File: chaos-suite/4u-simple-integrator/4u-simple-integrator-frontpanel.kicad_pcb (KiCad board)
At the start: 2 copper layers, 25 x 175 mm, 1 part

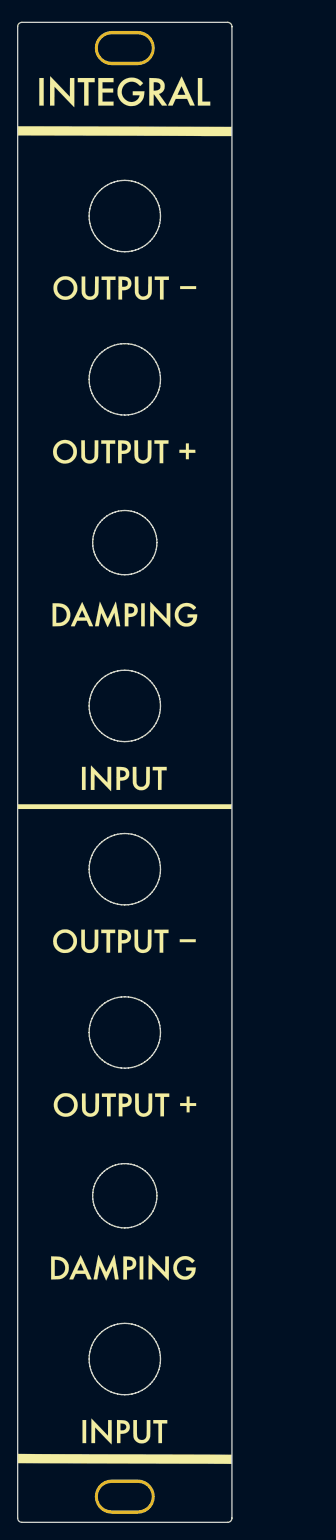
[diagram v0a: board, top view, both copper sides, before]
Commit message: Updating simple integrator to rev2
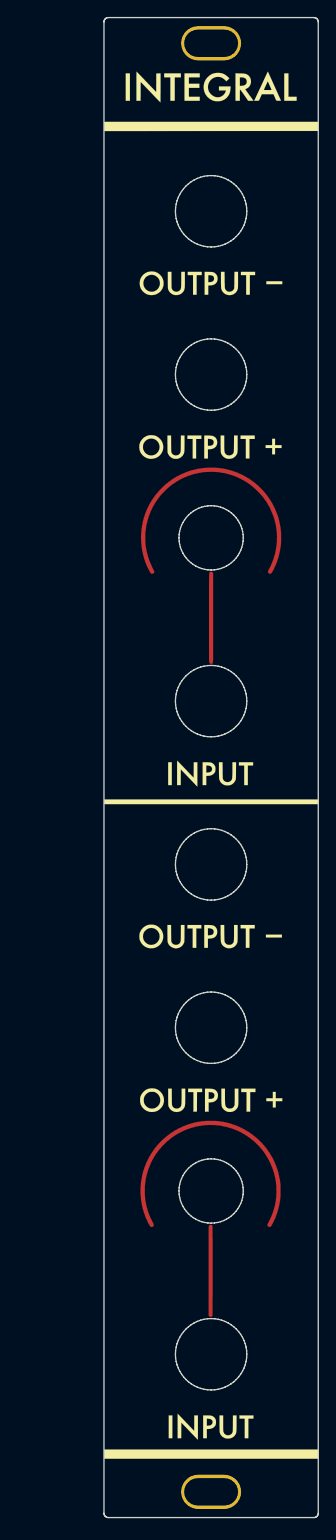
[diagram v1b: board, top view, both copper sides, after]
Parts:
- moved Ref** 88.1 mm to (72.5, 18.8)
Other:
- outline, holes or cut-outs redrawn
